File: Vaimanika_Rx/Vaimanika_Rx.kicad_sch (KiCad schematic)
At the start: 54 parts, among them T1 0900PC16J0042001E, U1 LR1121IMLTRT, U2 RFX2401C, U3 SKY13373-460LF, U4 ESP32-C3FH4, U5 TLV75533PDQNR, U6 OW2EL89CENUXFMYLC-32M, U7 ANT3216LL00R2400A, U8 TS2306A 240GF MSM 9_C2976675, X1 CJ17-400001010B20

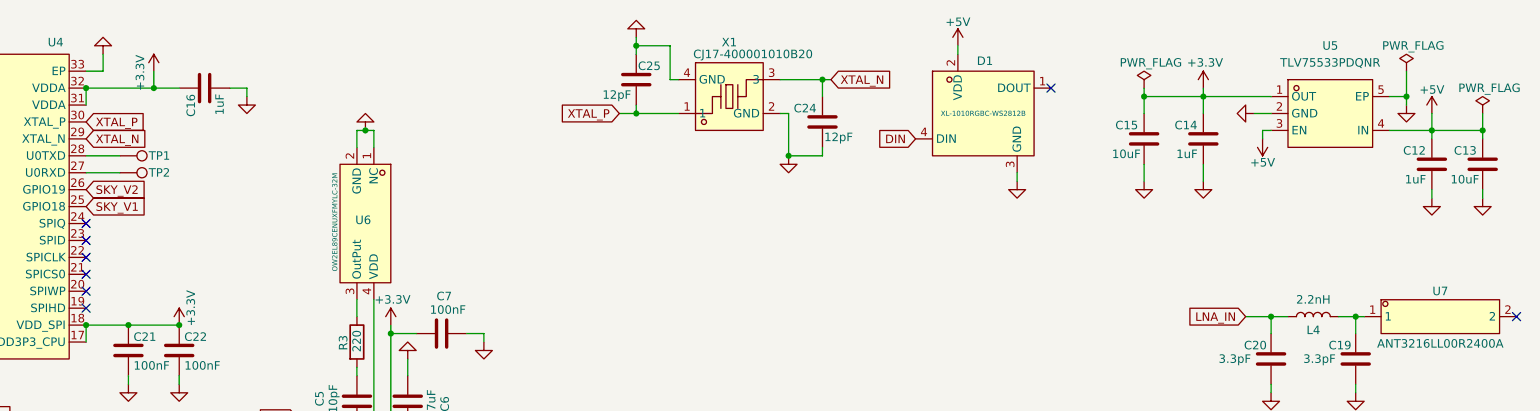
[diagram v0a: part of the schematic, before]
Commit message: 28-05-2026
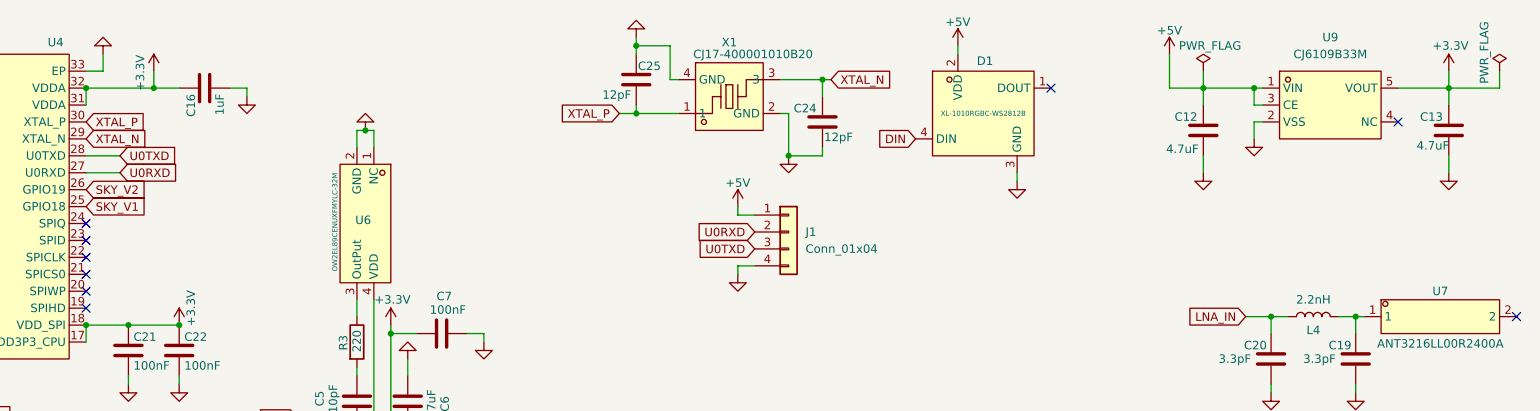
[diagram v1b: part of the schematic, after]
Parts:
- removed C14: 1uF, Capacitor_SMD:C_0402_1005Metric, symbol Device:C
- removed C15: 10uF, Capacitor_SMD:C_0402_1005Metric, symbol Device:C
- removed TP1, TP2: TestPoint, Connector_Wire:SolderWirePad_1x01_SMD_1x2mm, symbol Connector:TestPoint
- removed U5: TLV75533PDQNR, New_Library:X2SON-4_L1.0-W1.0-P0.65-TL-EP, symbol New_Library:TLV75533PDQNR
- added J1: Conn_01x04, New_Library:Rec_Conn_01x04, symbol Connector_Generic:Conn_01x04
- added U9: CJ6109B33M, New_Library:SOT-23-5_L2.9-W1.6-P0.95-LS2.8-BR, symbol New_Library:CJ6109B33M
- C12: value 1uF -> 4.7uF; LCSC C5137474 -> C22399610
- C13: value 10uF -> 4.7uF; LCSC C7472949 -> C22399610
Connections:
- net +3.3V: now also C13.1, U9.5 (VOUT)
- net +5V: now also J1.1 (Pin_1), U9.1 (VIN), U9.3 (CE); no longer C13.1
- net GND: now also J1.4 (Pin_4), U9.2 (VSS)
- net U0RXD: now reaches U4.27 (U0RXD)
- net U0RXD: now also J1.2 (Pin_2)
- net U0TXD: now reaches U4.28 (U0TXD)
- net U0TXD: now also J1.3 (Pin_3)
- no-connect marks 21 -> 22
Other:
- moved on the sheet: C12, C13
